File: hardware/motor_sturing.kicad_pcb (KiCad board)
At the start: 4 copper layers, 220 x 100 mm, 362 parts, among them CON1 BARREL_JACK, J1 DB25_STACKED, J2 ETHERNET_DUAL, M1 C3M0280090J, M10 C3M0280090J, M11 C3M0280090J, M12 C3M0280090J, M2 C3M0280090J, M3 C3M0280090J, M4 C3M0280090J, M5 C3M0280090J, M6 C3M0280090J, M7 C3M0280090J, M8 C3M0280090J, M9 C3M0280090J, P1 CONN_01X03, P10 CONN_01X01, P11 CONN_01X01, P12 CONN_01X01, P13 CONN_01X01, P14 CONN_01X01, P15 CONN_01X01, P16 CONN_01X01, P17 CONN_01X01, P18 CONN_01X01, P19 CONN_01X01, P2 CONN_01X03, P20 CONN_01X01, P21 CONN_01X01, P22 CONN_01X01, P23 CONN_01X01, P3 CONN_01X03, P4 CONN_01X03, P5 CONN_02X07, P6 CONN_01X01, P7 CONN_01X01, P8 CONN_01X01, P9 CONN_01X01, U1 LTC2351-14, U10 MAX3463, U11 MAX3463, U12 MAX3463, U13 MAX3463, U14 MAX3463, U15 Si8261BCD-C-IS, U16 TS321, U17 Si8261BCD-C-IS, U18 Si8261BCD-C-IS, U19 AD8226, U2 XC6SLXN-TQG144, U20 AD8226, U21 AD8226, U22 LTC2351-14, U23 LT3010, U24 Si8261BCD-C-IS, U25 AMC1204, U26 OKR_T3, U27 Si8261BCD-C-IS, U28 ACS722KMATR-20AB-T, U29 MAX3463, U3 W25Q80DV, U30 MAX3463, U31 MAX3463, U32 MAX3463, U33 MAX3463, U34 Si8261BCD-C-IS, U35 Si8261BCD-C-IS, U36 ACS722KMATR-20AB-T, U37 TS321, U38 AD8226, U39 AD8226, U4 KSZ9031RNXCA, U40 AD8226, U41 OKR_T3, U42 LT3010, U43 ACS722KMATR-20AB-T, U44 AMC1204, U45 OKR_T3, U46 TS321, U47 TS321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

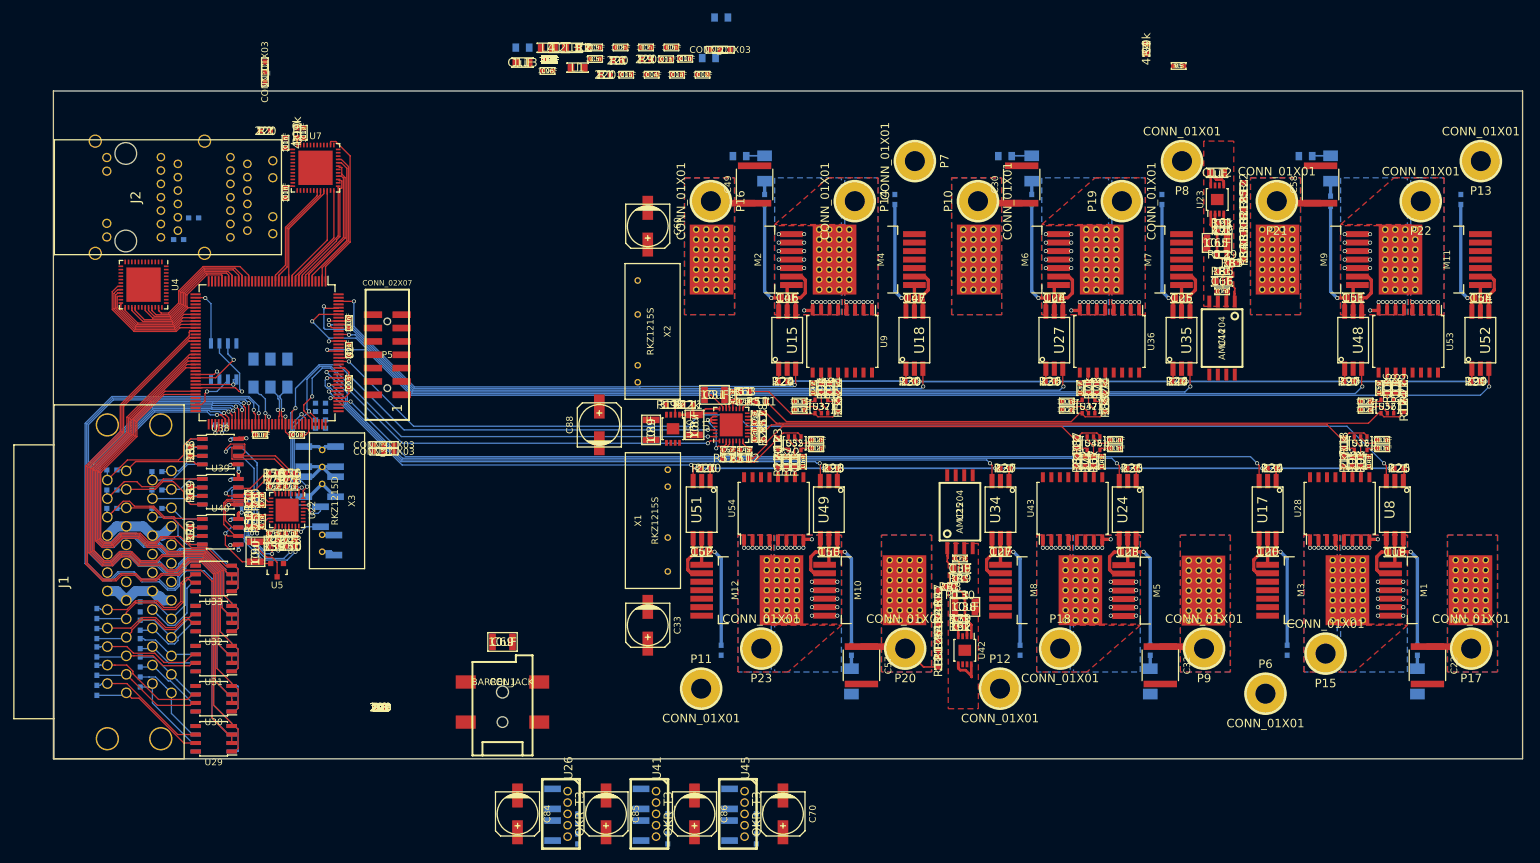
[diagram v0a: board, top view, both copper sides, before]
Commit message: Progress.
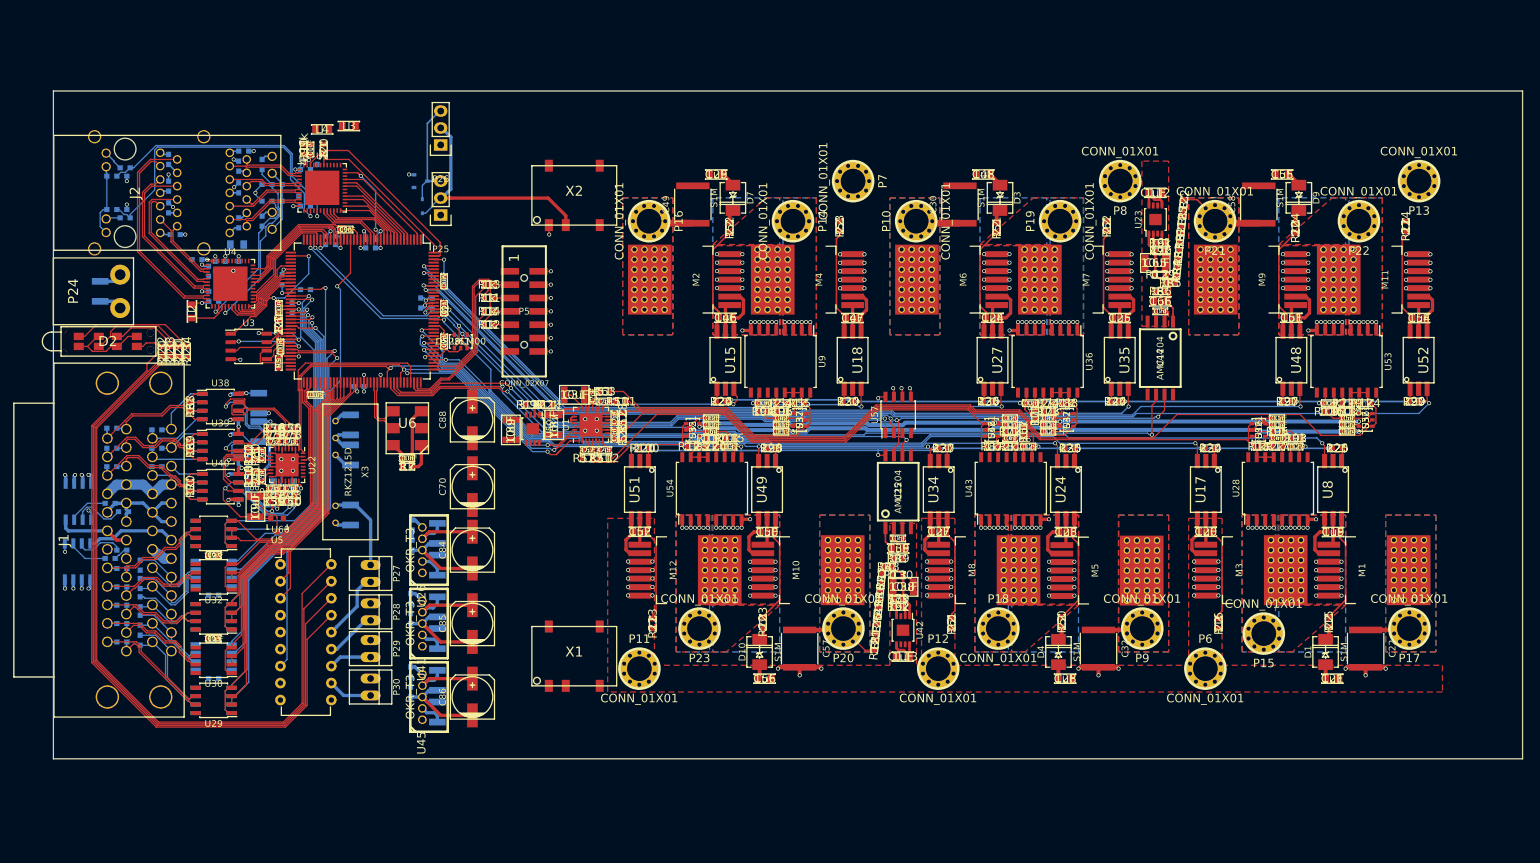
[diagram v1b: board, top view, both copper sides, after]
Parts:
- removed CON1: BARREL_JACK, 00_Passives:smd_barrel_jack
- added C126: 100nF, 00_Passives:C0603, F.Cu at (221.0, 96.8)
- added C127: 100nF, 00_Passives:C0603, F.Cu at (216.0, 103.2)
- added C128: 100nF, 00_Passives:C0603, F.Cu at (176.2, 96.8)
- added C129: 100nF, 00_Passives:C0603, F.Cu at (176.0, 103.2)
- added C130: 100nF, 00_Passives:C0603, F.Cu at (136.2, 96.8)
- added C131: 100nF, 00_Passives:C0603, F.Cu at (131.2, 103.2)
- added D2: LED_592, 00_Passives:LED_592-3030-013F, F.Cu at (38.1, 87.5)
- added D5: DIODE, Diodes_SMD:SOD-323, B.Cu at (85.2, 67.2)
- added M13: BSS138, 00_Passives:SOT23_GSD, B.Cu at (85.0, 63.5)
- added P24: CONN_01X02, 00_Passives:FCI_02_5mm, F.Cu at (40.0, 80.0)
- added P25: CONN_01X03, Pin_Headers:Pin_Header_Straight_1x03, F.Cu at (88.0, 68.6)
- added P26: CONN_01X03, Pin_Headers:Pin_Header_Straight_1x03, F.Cu at (88.0, 58.1)
- added P27: CONN_01X02, Connect:PINHEAD1-2, F.Cu at (77.5, 122.2)
- added P28: CONN_01X02, Connect:PINHEAD1-2, F.Cu at (77.5, 128.0)
- added P29: CONN_01X02, Connect:PINHEAD1-2, F.Cu at (77.5, 133.5)
- added P30: CONN_01X02, Connect:PINHEAD1-2, F.Cu at (77.5, 139.2)
- added R131: 220, 00_Passives:R0603, F.Cu at (48.8, 89.0)
- added R132: 220, 00_Passives:R0603, F.Cu at (46.2, 89.0)
- added R133: 220, 00_Passives:R0603, F.Cu at (47.5, 89.0)
- added R134: 220, 00_Passives:R0603, F.Cu at (50.0, 89.0)
- added R135: 15k, 00_Passives:R0603, B.Cu at (38.5, 111.8)
- added R136: 15k, 00_Passives:R0603, B.Cu at (40.2, 118.8)
- added R137: 4.7k, 00_Passives:R0603, B.Cu at (38.5, 120.0)
- added R138: 4.7k, 00_Passives:R0603, B.Cu at (40.5, 113.0)
- added U57: LM75, Housings_SOIC:SOIC-8_3.9x4.9mm_Pitch1.27mm, F.Cu at (156.5, 98.5)
- added U58: ips511g, Housings_SOIC:SOIC-8_3.9x4.9mm_Pitch1.27mm, B.Cu at (33.8, 111.5)
- added U59: ips511g, Housings_SOIC:SOIC-8_3.9x4.9mm_Pitch1.27mm, B.Cu at (33.6, 120.5)
- added U60: UCN5841A, Housings_DIP:DIP-18_W7.62mm, F.Cu at (64.0, 120.9)
- added U61: DS28CM00, 00_Passives:SOT23_5, F.Cu at (91.0, 87.5)
- C1, C10, C100, C101, C102, C103, C107, C11, C110, C111, C12, C13, C14, C15, C16, C18, C2, C5, C6, C69, C7, C8, C9, C92, C94, C95, C98, C99, L1, P1, P2, P3, P4, R2, R3, R4, R8, R9: moved to B.Cu
- C105, C21, C28, C29, C48, C55, C56, D1, D10, D3, D4, D7, D9, R103, R104, R11, R113, R114, R12, R13, R14, R15, R16, R50, R51, R52, R53, R61, R62, U3, U6: moved to F.Cu
- C33: value 100uF/16V -> 100nF; footprint Capacitors_SMD:c_elec_6.3x5.3 -> 00_Passives:C0603
- C60: value 100uF/16V -> 100nF; footprint Capacitors_SMD:c_elec_6.3x5.3 -> 00_Passives:C0603; moved to B.Cu
- P10, P11, P12, P13, P14, P15, P16, P17, P18, P19, P20, P21, P22, P23, P6, P7, P8, P9: footprint 00_Passives:conn_01x01_3mm -> 00_Passives:WE_9774080151R
- X1, X2: value RKZ1215S -> R2S-1215/H; footprint 00_Passives:RKZXXXXS -> 00_Passives:RECOM_R2S
- moved C21 153.7 mm to (221.5, 138.0), turned to 0 degrees
- moved R4 145.6 mm to (51.5, 75.2), turned to 180 degrees
- moved R5 141.9 mm to (63.8, 90.8), turned to 270 degrees
- moved C28 107.1 mm to (181.5, 138.0), turned to 0 degrees
- moved C113 105.6 mm to (157.2, 134.7), turned to 180 degrees
- moved C56 99.2 mm to (136.5, 138.0), turned to 0 degrees
- moved C60 93.9 mm to (54.0, 138.0), turned to 0 degrees
- moved R8 89.4 mm to (40.8, 61.5), turned to 180 degrees
- moved C1 88.0 mm to (47.2, 60.2), turned to 90 degrees
- moved C2 84.3 mm to (47.2, 64.2), turned to 90 degrees
- moved R9 81.5 mm to (40.7, 69.0)
- moved C6 77.7 mm to (54.0, 80.0), turned to 0 degrees
- moved R3 74.9 mm to (61.2, 69.5), turned to 90 degrees
- moved C7 73.6 mm to (53.3, 77.0), turned to 270 degrees
- moved C8 71.8 mm to (54.0, 81.5), turned to 0 degrees
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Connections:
- C33 pad 1: /Drive_1/ISOL_15V -> +3.3V
- C33 pad 2: /Drive_1/BRIDGE- -> GND
- C60 pad 1: /Drive_2/ISOL_15V -> +3.3V
- C60 pad 2: /Drive_2/BRIDGE- -> GND
- C80 pad 1: +3V3 -> +3.3V
- C85 pad 1: +3V3 -> +3.3V
- J1 pad A20: +12V -> Net-(J1-PadA20)
- J1 pad A7: +12V -> Net-(J1-PadA20)
- J1 pad B20: +12V -> Net-(J1-PadB20)
- J1 pad B7: +12V -> Net-(J1-PadB20)
- J2 pad 10: /FPGA/TRXD0_P -> /FPGA/TRXC0_P
- J2 pad 11: /FPGA/TRXA0_N -> /FPGA/TRXB0_N
- J2 pad 12: Net-(C4-Pad1) -> Net-(C3-Pad1)
- J2 pad 13: /FPGA/TRXB0_P -> /FPGA/TRXA0_P
- J2 pad 2: /FPGA/TRXC0_P -> /FPGA/TRXD0_P
- J2 pad 3: /FPGA/TRXD0_N -> /FPGA/TRXC0_N
- J2 pad 4: Net-(C1-Pad1) -> Net-(C2-Pad1)
- J2 pad 5: /FPGA/TRXA0_P -> /FPGA/TRXB0_P
- J2 pad 6: /FPGA/TRXB0_N -> /FPGA/TRXA0_N
- J2 pad 7: Net-(C3-Pad1) -> Net-(C4-Pad1)
- J2 pad 8: /FPGA/TRXC0_N -> /FPGA/TRXD0_N
- J2 pad 9: Net-(C2-Pad1) -> Net-(C1-Pad1)
- R115 pad 1: +3V3 -> +3.3V
- R116 pad 1: +3V3 -> +3.3V
- R67 pad 1: +3V3 -> +3.3V
- R71 pad 1: +3V3 -> +3.3V
- R93 pad 1: +3V3 -> +3.3V
- R94 pad 1: +3V3 -> +3.3V
- U1 pad 26: +3V3 -> +3.3V
- U1 pad 27: +3V3 -> +3.3V
- U1 pad 28: +3V3 -> +3.3V
- U1 pad 3: +3V3 -> +3.3V
- U1 pad 33: (no net) -> GND
- U2 pad 102: /FPGA/SD1 -> /FPGA/SCK
- U2 pad 105: /FPGA/SCK -> /FPGA/SD1
- U2 pad 132: /FPGA/HB_L4 -> /Drive_2/H2
- U2 pad 134: /FPGA/HB_L3 -> /FPGA/HB_L4
- U2 pad 138: /Drive_2/H2 -> /Drive_2/H1
- U2 pad 140: /Drive_2/H1 -> /FPGA/HB_L3
- U2 pad 22: Net-(U2-Pad22) -> /FPGA/AUX_STR
- U2 pad 33: Net-(U2-Pad33) -> /FPGA/SCL
- U2 pad 34: Net-(U2-Pad34) -> /FPGA/SDA
- U2 pad 48: /Drive_2/ENC_DIR4 -> /Drive_1/ENC_DIR3
- U2 pad 50: /Drive_2/ENC_DATA4 -> /Drive_1/ENC_DATA0
- U2 pad 51: /Drive_2/ENC_DIR3 -> /Drive_1/ENC_DIR0
- U2 pad 55: /Drive_2/ENC_DATA3 -> /Drive_1/ENC_DATA1
- U2 pad 56: /Drive_2/ENC_DIR2 -> /Drive_1/ENC_DIR1
- U2 pad 57: /Drive_2/ENC_DATA2 -> /Drive_1/ENC_DATA2
- U2 pad 58: /Drive_2/ENC_DIR1 -> /Drive_1/ENC_DIR2
- U2 pad 59: /Drive_2/ENC_DATA1 -> /Drive_1/ENC_DATA3
- U2 pad 66: /Drive_2/ENC_DIR0 -> /Drive_1/ENC_DATA4
- U2 pad 67: /Drive_2/ENC_DATA0 -> /Drive_1/ENC_DIR4
- U2 pad 74: Net-(U2-Pad74) -> /Drive_2/ENC_DATA0
- U2 pad 75: Net-(U2-Pad75) -> /Drive_2/ENC_DIR0
- U2 pad 78: /Drive_1/ENC_DATA0 -> /Drive_2/ENC_DATA1
- U2 pad 79: /Drive_1/ENC_DIR0 -> /Drive_2/ENC_DIR1
- U2 pad 80: /Drive_1/ENC_DATA1 -> /Drive_2/ENC_DATA2
- U2 pad 81: /Drive_1/ENC_DIR1 -> /Drive_2/ENC_DIR2
- U2 pad 82: /Drive_1/ENC_DATA2 -> /Drive_2/ENC_DATA3
- U2 pad 83: /Drive_1/ENC_DIR2 -> /Drive_2/ENC_DIR3
- U2 pad 84: /Drive_1/ENC_DATA3 -> /Drive_2/ENC_DATA4
- U2 pad 85: /Drive_1/ENC_DIR3 -> /Drive_2/ENC_DIR4
- U2 pad 87: /Drive_1/ENC_DATA4 -> /FPGA/AUX_CLK
- U2 pad 88: /Drive_1/ENC_DIR4 -> /FPGA/AUX_DATA
- U2 pad 92: Net-(U2-Pad92) -> /FPGA/FAN
- U22 pad 26: +3V3 -> +3.3V
- U22 pad 27: +3V3 -> +3.3V
- U22 pad 28: +3V3 -> +3.3V
- U22 pad 3: +3V3 -> +3.3V
- U22 pad 33: (no net) -> GND
- U28 pad 10: +3V3 -> +3.3V
- U36 pad 10: +3V3 -> +3.3V
- U4 pad 2: /FPGA/TRXA0_N -> /FPGA/TRXA0_P
- U4 pad 3: /FPGA/TRXA0_P -> /FPGA/TRXA0_N
- U4 pad 49: (no net) -> GND
- U4 pad 5: /FPGA/TRXB0_N -> /FPGA/TRXB0_P
- U4 pad 6: /FPGA/TRXB0_P -> /FPGA/TRXB0_N
- U4 pad 7: /FPGA/TRXC0_N -> /FPGA/TRXC0_P
- U4 pad 8: /FPGA/TRXC0_P -> /FPGA/TRXC0_N
- U41 pad 4: +3V3 -> +3.3V
- U43 pad 10: +3V3 -> +3.3V
- U5 pad 1: +3V3 -> +3.3V
- U53 pad 10: +3V3 -> +3.3V
- U54 pad 10: +3V3 -> +3.3V
- U7 pad 49: (no net) -> GND
- U9 pad 10: +3V3 -> +3.3V
- X1 pad 5: /Drive_1/BRIDGE- -> /Drive_1/ISOL_15V
- X2 pad 5: /Drive_2/BRIDGE- -> /Drive_2/ISOL_15V
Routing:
- net GND: track 87.2 -> 304.6 mm, vias 7 -> 58
- net +5V: track 9.92 -> 142.0 mm, vias 0 -> 6
- net /Drive_1/VOLTAGE_CLOCK: track 0.00 -> 128.7 mm, vias 0 -> 3
- net /FPGA/VOLTAGE_D1: track 0.00 -> 125.8 mm, vias 0 -> 2
- net Net-(R134-Pad2): track 0.00 -> 111.1 mm
- net -5V: track 19.1 -> 127.2 mm, vias 0 -> 6
- net Net-(R133-Pad2): track 0.00 -> 107.1 mm
- net Net-(R131-Pad2): track 0.00 -> 106.4 mm
- net /FPGA/SCL: track 0.00 -> 105.7 mm, vias 0 -> 3
- net Net-(R132-Pad2): track 0.00 -> 104.5 mm
- net /FPGA/SDA: track 0.00 -> 104.1 mm, vias 0 -> 3
- net /FPGA/VOLTAGE_D0: track 0.00 -> 85.5 mm, vias 0 -> 2
- net /Drive_1/BRIDGE-: track 1.60 -> 79.3 mm, vias 0 -> 39
- net +12V: track 2.02 -> 78.8 mm, vias 0 -> 8
- net +3.3V: track 229.1 -> 301.9 mm, vias 13 -> 25
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- added copper zone on In2.Cu, net +12V
- added copper zone on In1.Cu, net /Drive_1/BRIDGE-
- added copper zone on In1.Cu, net /Drive_2/BRIDGE-
- added copper zone on In1.Cu, net GND
